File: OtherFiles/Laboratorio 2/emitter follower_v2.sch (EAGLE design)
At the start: 3 parts

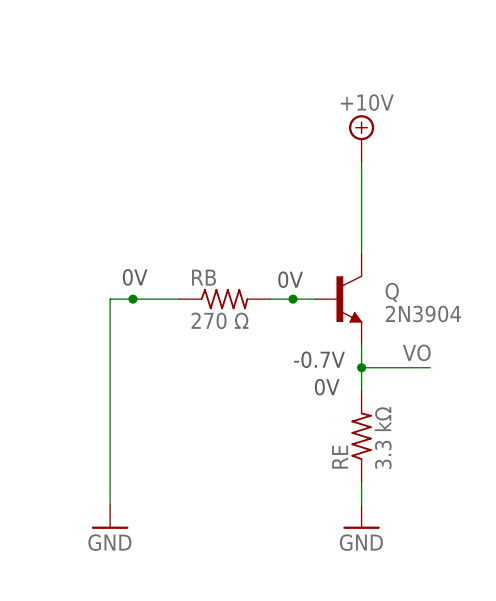
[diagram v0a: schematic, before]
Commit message: continuata analisi laboratorio 2
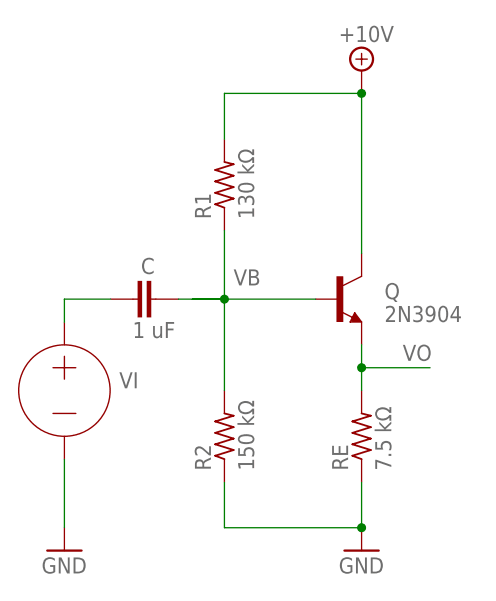
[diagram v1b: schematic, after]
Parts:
- removed RB: 270 Ω, rcl:R-US_0204/5
- added C: 1 uF, rcl:C-EU025-030X050
- added R1: 130 kΩ, rcl:R-US_0204/5
- added R2: 150 kΩ, rcl:R-US_0204/5
- added VI: 0V, ngspice-simulation:VOLTAGE
- RE: value 3.3 kΩ -> 7.5 kΩ
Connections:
- new net N$1: Q.B
- new net N$3: C.2, R1.1, R2.2
- net +10V: now also R1.2
- net GND: now also R2.1, VI.-; no longer RB.1
- net N$2: now also C.1, VI.+; no longer Q.B, RB.2
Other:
- note added: "VB"
- note removed: "-0.7V"
- note removed: "0V"
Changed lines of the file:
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@@
 <parts>
 <part name="Q" library="transistor" library_urn="urn:adsk.eagle:library:402" deviceset="2N3904" device="" package3d_urn="urn:adsk.eagle:package:28523/2"/>
-<part name="RB" library="rcl" library_urn="urn:adsk.eagle:library:334" deviceset="R-US_" device="0204/5" package3d_urn="urn:adsk.eagle:package:23488/1" value="270 Ω"/>
-<part name="RE" library="rcl" library_urn="urn:adsk.eagle:library:334" deviceset="R-US_" device="0204/5" package3d_urn="urn:adsk.eagle:package:23488/1" value="3.3 kΩ"/>
+<part name="VI" library="ngspice-simulation" library_urn="urn:adsk.eagle:library:527439" deviceset="VOLTAGE" device="" value="0V"/>
+<part name="RE" library="rcl" library_urn="urn:adsk.eagle:library:334" deviceset="R-US_" device="0204/5" package3d_urn="urn:adsk.eagle:package:23488/1" value="7.5 kΩ"/>
 <part name="GND1" library="supply1" library_urn="urn:adsk.eagle:library:371" deviceset="GND" device=""/>
 <part name="SUPPLY1" library="supply2" library_urn="urn:adsk.eagle:library:372" deviceset="+10V" device=""/>
 <part name="GND2" library="supply1" library_urn="urn:adsk.eagle:library:371" deviceset="GND" device=""/>
+<part name="R1" library="rcl" library_urn="urn:adsk.eagle:library:334" deviceset="R-US_" device="0204/5" package3d_urn="urn:adsk.eagle:package:23488/1" value="130 kΩ"/>
+<part name="R2" library="rcl" library_urn="urn:adsk.eagle:library:334" deviceset="R-US_" device="0204/5" package3d_urn="urn:adsk.eagle:package:23488/1" value="150 kΩ"/>
+<part name="C" library="rcl" library_urn="urn:adsk.eagle:library:334" deviceset="C-EU" device="025-030X050" package3d_urn="urn:adsk.eagle:package:23631/1" value="1 uF"/>
 </parts>
 <sheets>
 <sheet>
 <plain>
-<text x="29.21" y="42.164" size="1.778" layer="92">0V</text>
-<text x="46.482" y="41.91" size="1.778" layer="92">0V</text>
-<text x="48.26" y="33.02" size="1.778" layer="92">-0.7V</text>
-<text x="50.546" y="29.972" size="1.778" layer="92">0V</text>
+<text x="41.656" y="42.164" size="1.778" layer="95">VB</text>
 </plain>
 <instances>
@@
 <attribute name="VALUE" x="58.42" y="38.1" size="1.778" layer="96"/>
 </instance>
-<instance part="RB" gate="G$1" x="40.64" y="40.64" smashed="yes">
-<attribute name="NAME" x="36.83" y="42.1386" size="1.778" layer="95"/>
-<attribute name="VALUE" x="36.83" y="37.338" size="1.778" layer="96"/>
+<instance part="VI" gate="G$1" x="22.86" y="30.48" smashed="yes">
+<attribute name="NAME" x="28.956" y="30.734" size="1.778" layer="95"/>
 </instance>
 <instance part="RE" gate="G$1" x="55.88" y="25.4" smashed="yes" rot="R90">
@@
 <attribute name="VALUE" x="59.182" y="21.59" size="1.778" layer="96" rot="R90"/>
 </instance>
-<instance part="GND1" gate="1" x="27.94" y="15.24" smashed="yes">
-<attribute name="VALUE" x="25.4" y="12.7" size="1.778" layer="96"/>
+<instance part="GND1" gate="1" x="22.86" y="12.7" smashed="yes">
+<attribute name="VALUE" x="20.32" y="10.16" size="1.778" layer="96"/>
 </instance>
-<instance part="SUPPLY1" gate="G$1" x="55.88" y="58.42" smashed="yes">
-<attribute name="VALUE" x="53.34" y="61.595" size="1.778" layer="96"/>
+<instance part="SUPPLY1" gate="G$1" x="55.88" y="66.04" smashed="yes">
+<attribute name="VALUE" x="53.34" y="69.215" size="1.778" layer="96"/>
 </instance>
-<instance part="GND2" gate="1" x="55.88" y="15.24" smashed="yes">
-<attribute name="VALUE" x="53.34" y="12.7" size="1.778" layer="96"/>
+<instance part="GND2" gate="1" x="55.88" y="12.7" smashed="yes">
+<attribute name="VALUE" x="53.34" y="10.16" size="1.778" layer="96"/>
+</instance>
+<instance part="R1" gate="G$1" x="40.64" y="53.34" smashed="yes" rot="R90">
+<attribute name="NAME" x="39.1414" y="49.53" size="1.778" layer="95" rot="R90"/>
+<attribute name="VALUE" x="43.942" y="49.53" size="1.778" layer="96" rot="R90"/>
+</instance>
+<instance part="R2" gate="G$1" x="40.64" y="25.4" smashed="yes" rot="R90">
+<attribute name="NAME" x="39.1414" y="21.59" size="1.778" layer="95" rot="R90"/>
+<attribute name="VALUE" x="43.942" y="21.59" size="1.778" layer="96" rot="R90"/>
+</instance>
+<instance part="C" gate="G$1" x="30.48" y="40.64" smashed="yes" rot="R90">
+<attribute name="NAME" x="32.893" y="45.212" size="1.778" layer="95" rot="R180"/>
+<attribute name="VALUE" x="35.179" y="38.1" size="1.778" layer="96" rot="R180"/>
 </instance>
 </instances>
@@
 </segment>
 </net>
-<net name="N$2" class="0">
+<net name="N$3" class="0">
 <segment>
-<pinref part="Q" gate="G1" pin="B"/>
-<pinref part="RB" gate="G$1" pin="2"/>
-<wire x1="50.8" y1="40.64" x2="48.26" y2="40.64" width="0.1524" layer="91"/>
-<junction x="48.26" y="40.64"/>
-<wire x1="48.26" y1="40.64" x2="45.72" y2="40.64" width="0.1524" layer="91"/>
+<pinref part="R1" gate="G$1" pin="1"/>
+<pinref part="R2" gate="G$1" pin="2"/>
+<wire x1="40.64" y1="48.26" x2="40.64" y2="40.64" width="0.1524" layer="91"/>
+<wire x1="40.64" y1="40.64" x2="40.64" y2="30.48" width="0.1524" layer="91"/>
+<wire x1="37.084" y1="40.64" x2="40.64" y2="40.64" width="0.1524" layer="91"/>
+<junction x="40.64" y="40.64"/>
+<pinref part="C" gate="G$1" pin="2"/>
+<wire x1="35.56" y1="40.64" x2="40.64" y2="40.64" width="0.1524" layer="91"/>
 </segment>
 </net>
 <net name="GND" class="0">
 <segment>
+<pinref part="VI" gate="G$1" pin="-"/>
 <pinref part="GND1" gate="1" pin="GND"/>
-<pinref part="RB" gate="G$1" pin="1"/>
-<wire x1="27.94" y1="40.64" x2="30.48" y2="40.64" width="0.1524" layer="91"/>
-<wire x1="30.48" y1="40.64" x2="35.56" y2="40.64" width="0.1524" layer="91"/>
-<wire x1="27.94" y1="40.64" x2="27.94" y2="17.78" width="0.1524" layer="91"/>
-<junction x="30.48" y="40.64"/>
+<wire x1="22.86" y1="22.86" x2="22.86" y2="15.24" width="0.1524" layer="91"/>
 </segment>
 <segment>
 <pinref part="RE" gate="G$1" pin="1"/>
-<wire x1="55.88" y1="17.78" x2="55.88" y2="20.32" width="0.1524" layer="91"/>
+<wire x1="55.88" y1="15.24" x2="55.88" y2="20.32" width="0.1524" layer="91"/>
 <pinref part="GND2" gate="1" pin="GND"/>
+<pinref part="R2" gate="G$1" pin="1"/>
+<wire x1="40.64" y1="20.32" x2="40.64" y2="15.24" width="0.1524" layer="91"/>
+<wire x1="40.64" y1="15.24" x2="55.88" y2="15.24" width="0.1524" layer="91"/>
+<junction x="55.88" y="15.24"/>
 </segment>
 </net>
@@
 <segment>
 <pinref part="Q" gate="G1" pin="C"/>
-<wire x1="55.88" y1="45.72" x2="55.88" y2="55.88" width="0.1524" layer="91"/>
+<wire x1="55.88" y1="45.72" x2="55.88" y2="63.5" width="0.1524" layer="91"/>
 <pinref part="SUPPLY1" gate="G$1" pin="+10V"/>
+<wire x1="55.88" y1="63.5" x2="40.64" y2="63.5" width="0.1524" layer="91"/>
+<junction x="55.88" y="63.5"/>
+<pinref part="R1" gate="G$1" pin="2"/>
+<wire x1="40.64" y1="63.5" x2="40.64" y2="58.42" width="0.1524" layer="91"/>
 </segment>
 </net>
+<net name="N$1" class="0">
+<segment>
+<pinref part="Q" gate="G1" pin="B"/>
+<wire x1="39.624" y1="40.64" x2="50.8" y2="40.64" width="0.1524" layer="91"/>
+</segment>
+</net>
+<net name="N$2" class="0">
+<segment>
+<pinref part="VI" gate="G$1" pin="+"/>
+<pinref part="C" gate="G$1" pin="1"/>
+<wire x1="22.86" y1="38.1" x2="22.86" y2="40.64" width="0.1524" layer="91"/>
+<wire x1="22.86" y1="40.64" x2="27.94" y2="40.64" width="0.1524" layer="91"/>
+</segment>
+</net>
